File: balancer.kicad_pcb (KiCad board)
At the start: 2 copper layers, 50 x 50 mm, 53 parts, among them IC1 TLV3404, IC2 MAX923, IC3 MAX923, IC4 MAX923, J1 S4B-XH-SM4-TB, J2 Output (+), J3 Output (-), J4 Input (+), J5 Input (-), Q1 IRF7455PBF, Q2 IRF7455PBF, Q3 IRF7455PBF, Q4 IRF7455PBF

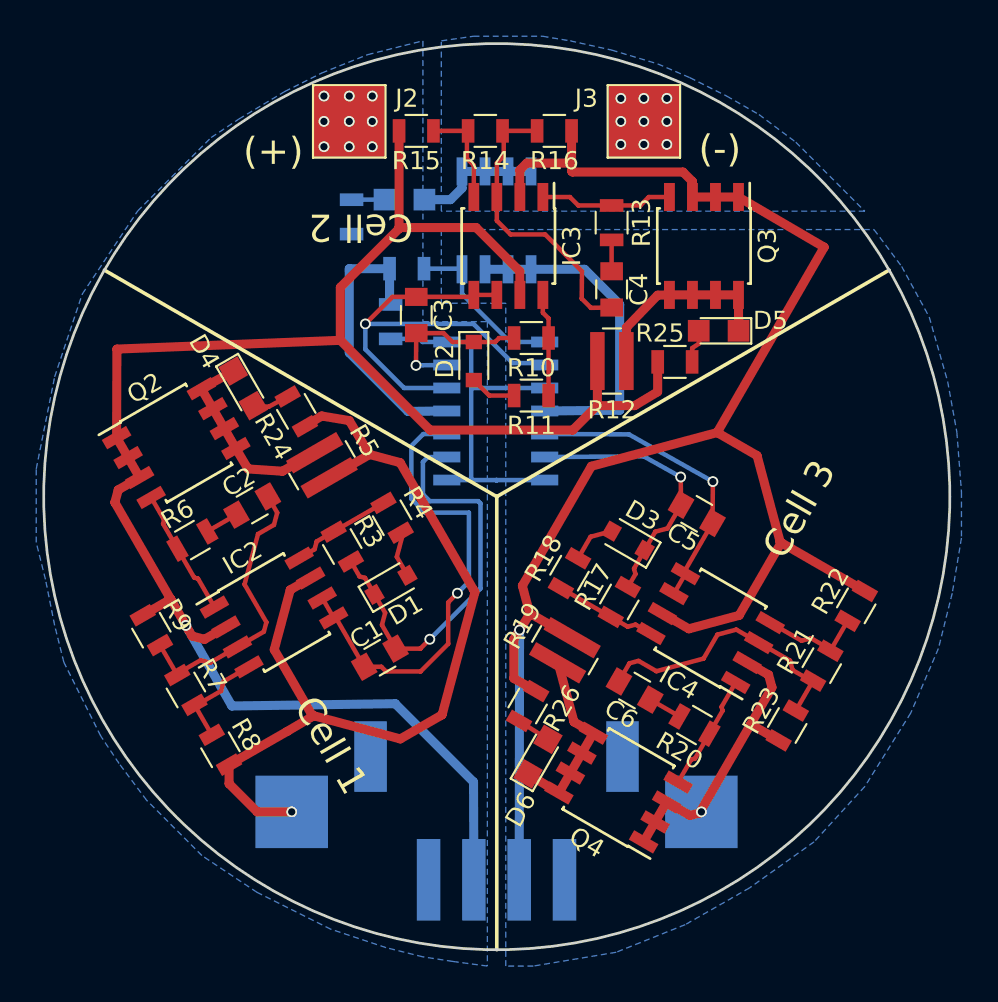
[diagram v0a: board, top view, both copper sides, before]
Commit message: final version sent off to board manufacturer
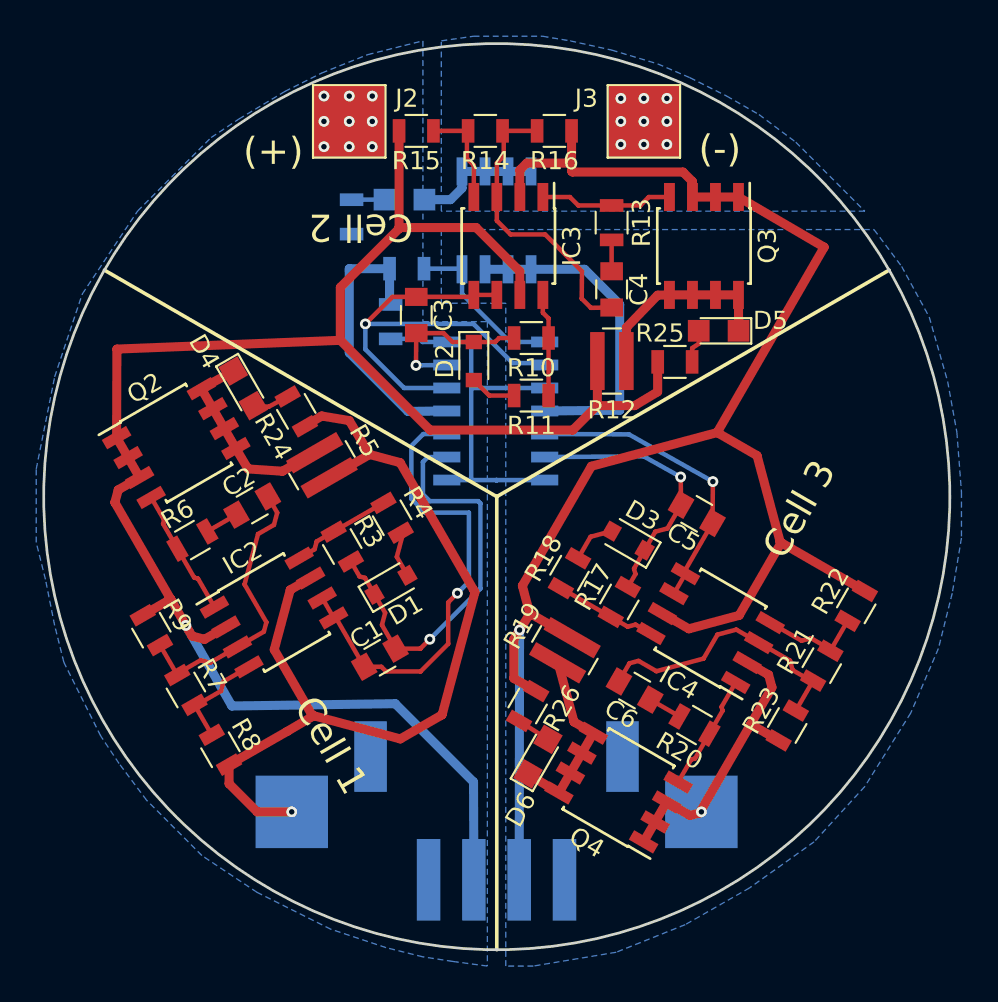
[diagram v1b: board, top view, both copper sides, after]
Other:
- net class Default: via_drill 0.4 -> 0.3
- net class Power: via_drill 0.4 -> 0.3
- rule via_min_size: 0.4 -> 0.3
